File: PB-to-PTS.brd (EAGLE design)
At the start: 111.8 x 38.1 mm, 8 parts, among them J1 PulseBlaster, J3 PTS-PORT

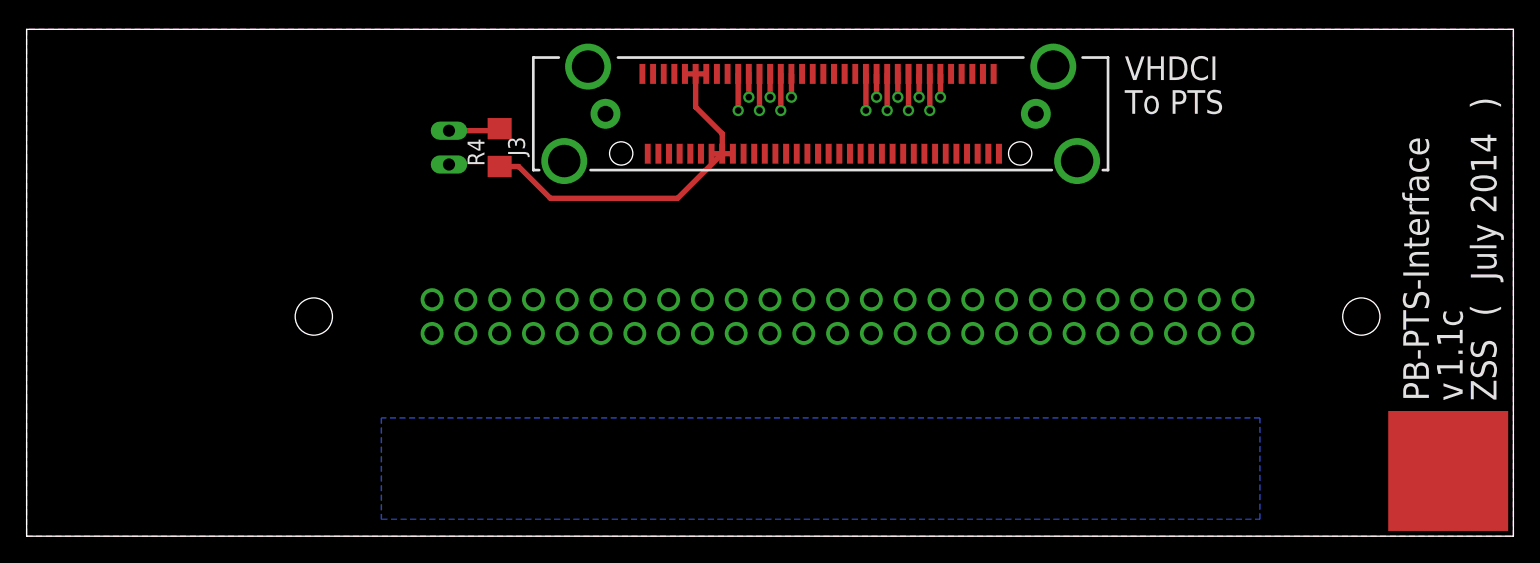
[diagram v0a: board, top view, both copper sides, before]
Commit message: Clean up schematic, route board
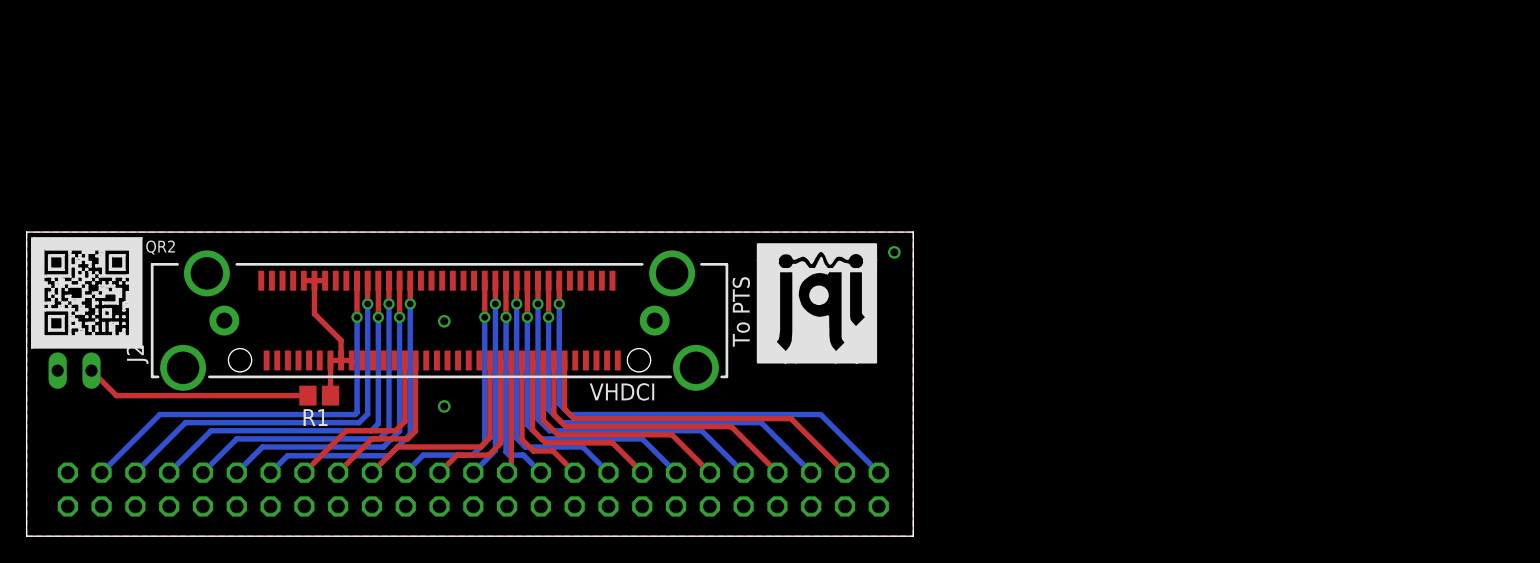
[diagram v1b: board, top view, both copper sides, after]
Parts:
- removed J1: PulseBlaster, PTS_Board_Lib:09185505909
- removed J3: PTS-PORT, PTS_Board_Lib:MOLEX-73776-0201
- removed R4: ~200R, resistor:R1206
- removed U$6: (no value), PTS_Board_Lib:INFO_BLOCK-0.076
- added J2: PTS-PORT, PTS_Board_Lib:MOLEX-73776-0201
- added LED: LED, jumper:JP1
- added QR1, QR2: QR-HTTP://GIT.IO/VC0XU, QR-git.io-vc0xU:QR-HTTP://GIT.IO/VC0XU
- added R1: ~200R, resistor:R0805
- JP1: value LED -> (none); device jumper:JP1 -> pinhead:2X25
- U$3: device JQI_Logo:JQI_LOGO_NEGATIVE-COPPER -> JQI_Logo:JQI_LOGO_NEGATIVE-SILKSCREEN
- moved U$2 60.6 mm to (43.6, 7.57), turned to 0 degrees
- moved U$3 57.7 mm to (55.0, 13.1), turned to 0 degrees
- moved U$4 40.7 mm to (63.9, 13.1), turned to 0 degrees
- moved JP1 25.8 mm to (33.6, 3.51)
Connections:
- net AGND: now also J2.26; no longer J3.26
- net GND: now also J2.56, J2.64, J2.SHIELD1, J2.SHIELD2, J2.SHIELD3, J2.SHIELD4, J2.SHIELD5, J2.SHIELD6, JP1.11, JP1.13, JP1.15, JP1.17, JP1.19, JP1.21, JP1.23, JP1.25, JP1.27, JP1.29, JP1.3, JP1.31, JP1.33, JP1.35, JP1.37, JP1.39, JP1.41, JP1.43, JP1.45, JP1.47, JP1.49, JP1.5, JP1.7, JP1.9, LED.1; no longer J1.1, J1.11, J1.13, J1.15, J1.17, J1.19, J1.21, J1.23, J1.25, J1.27, J1.29, J1.3, J1.31, J1.33, J1.35, J1.37, J1.39, J1.41, J1.43, J1.45, J1.47, J1.49, J1.5, J1.7, J1.9, J3.56, J3.64, J3.SHIELD1, J3.SHIELD2, J3.SHIELD3, J3.SHIELD4, J3.SHIELD5, J3.SHIELD6
- net N$3: now also LED.2, R1.2; no longer JP1.2, R4.2
- net PB0: now also J2.6, JP1.2; no longer J1.2, J3.6
- net PB1: now also J2.40, JP1.4; no longer J1.4, J3.40
- net PB10: now also J2.11, JP1.22; no longer J1.22, J3.11
- net PB11: now also J2.45, JP1.24; no longer J1.24, J3.45
- net PB12: now also J2.12, JP1.26; no longer J1.26, J3.12
- net PB13: now also J2.46, JP1.28; no longer J1.28, J3.46
- net PB14: now also J2.13, JP1.30; no longer J1.30, J3.13
- net PB15: now also J2.47, JP1.32; no longer J1.32, J3.47
- net PB16: now also J2.54, JP1.34; no longer J1.34, J3.54
- net PB17: now also J2.55, JP1.36; no longer J1.36, J3.55
- net PB18: now also J2.20, JP1.38; no longer J1.38, J3.20
- net PB19: now also J2.21, JP1.40; no longer J1.40, J3.21
- net PB2: now also J2.7, JP1.6; no longer J1.6, J3.7
- net PB20: now also J2.22, JP1.42; no longer J1.42, J3.22
- net PB21: now also J2.23, JP1.44; no longer J1.44, J3.23
- net PB22: now also J2.24, JP1.46; no longer J1.46, J3.24
- net PB23: now also J2.25, JP1.48; no longer J1.48, J3.25
- net PB3: now also J2.41, JP1.8; no longer J1.8, J3.41
- net PB4: now also J2.8, JP1.10; no longer J1.10, J3.8
- net PB5: now also J2.42, JP1.12; no longer J1.12, J3.42
- net PB6: now also J2.9, JP1.14; no longer J1.14, J3.9
- net PB7: now also J2.43, JP1.16; no longer J1.16, J3.43
- net PB8: now also J2.10, JP1.18; no longer J1.18, J3.10
- net PB9: now also J2.44, JP1.20; no longer J1.20, J3.44
- net PTS+5V: now also J2.28, J2.29, J2.30, J2.60, J2.61, J2.62, R1.1; no longer J3.28, J3.29, J3.30, J3.60, J3.61, J3.62, R4.1
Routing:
- net PB0: track 1.75 -> 35.4 mm
- net PB2: track 2.75 -> 31.4 mm
- net PB23: track 2.75 -> 31.0 mm
- net PB22: track 1.75 -> 29.3 mm
- net PB1: track 0.00 -> 26.7 mm
- net PB4: track 1.75 -> 27.5 mm
- net PB21: track 2.75 -> 28.0 mm
- net PB20: track 1.75 -> 26.5 mm
- net PB3: track 0.00 -> 22.7 mm
- net PB19: track 2.75 -> 24.8 mm
- net PB18: track 1.75 -> 23.2 mm
- net PB6: track 2.75 -> 23.5 mm
- net PB5: track 0.00 -> 18.6 mm
- net PB8: track 1.75 -> 19.8 mm
- net PTS+5V: track 29.1 -> 12.7 mm
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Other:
- board size 111.8 x 38.1 mm -> 66.6 x 22.9 mm
